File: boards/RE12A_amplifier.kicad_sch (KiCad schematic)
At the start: 14 parts, among them J14 RE12A, J15 Conn_01x03 encoder_direct, Q1 NPN, U3 MOUDLE-SEEEDUINO-XIAO-ESP32C3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, U7 LM397

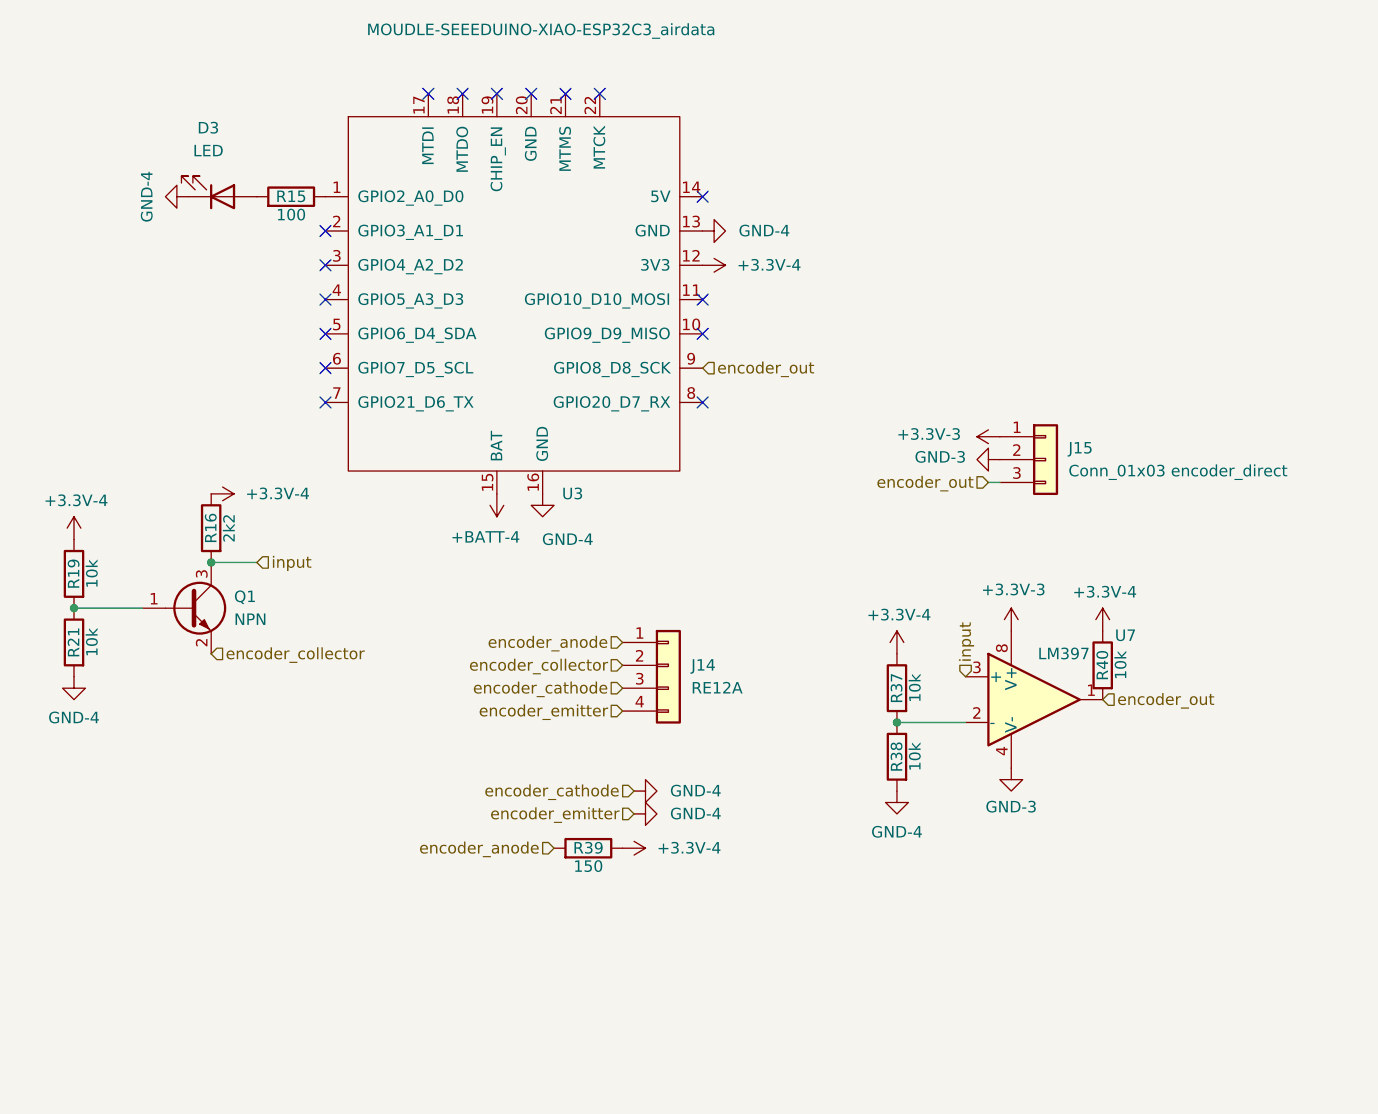
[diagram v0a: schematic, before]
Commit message: DRCエラー解消
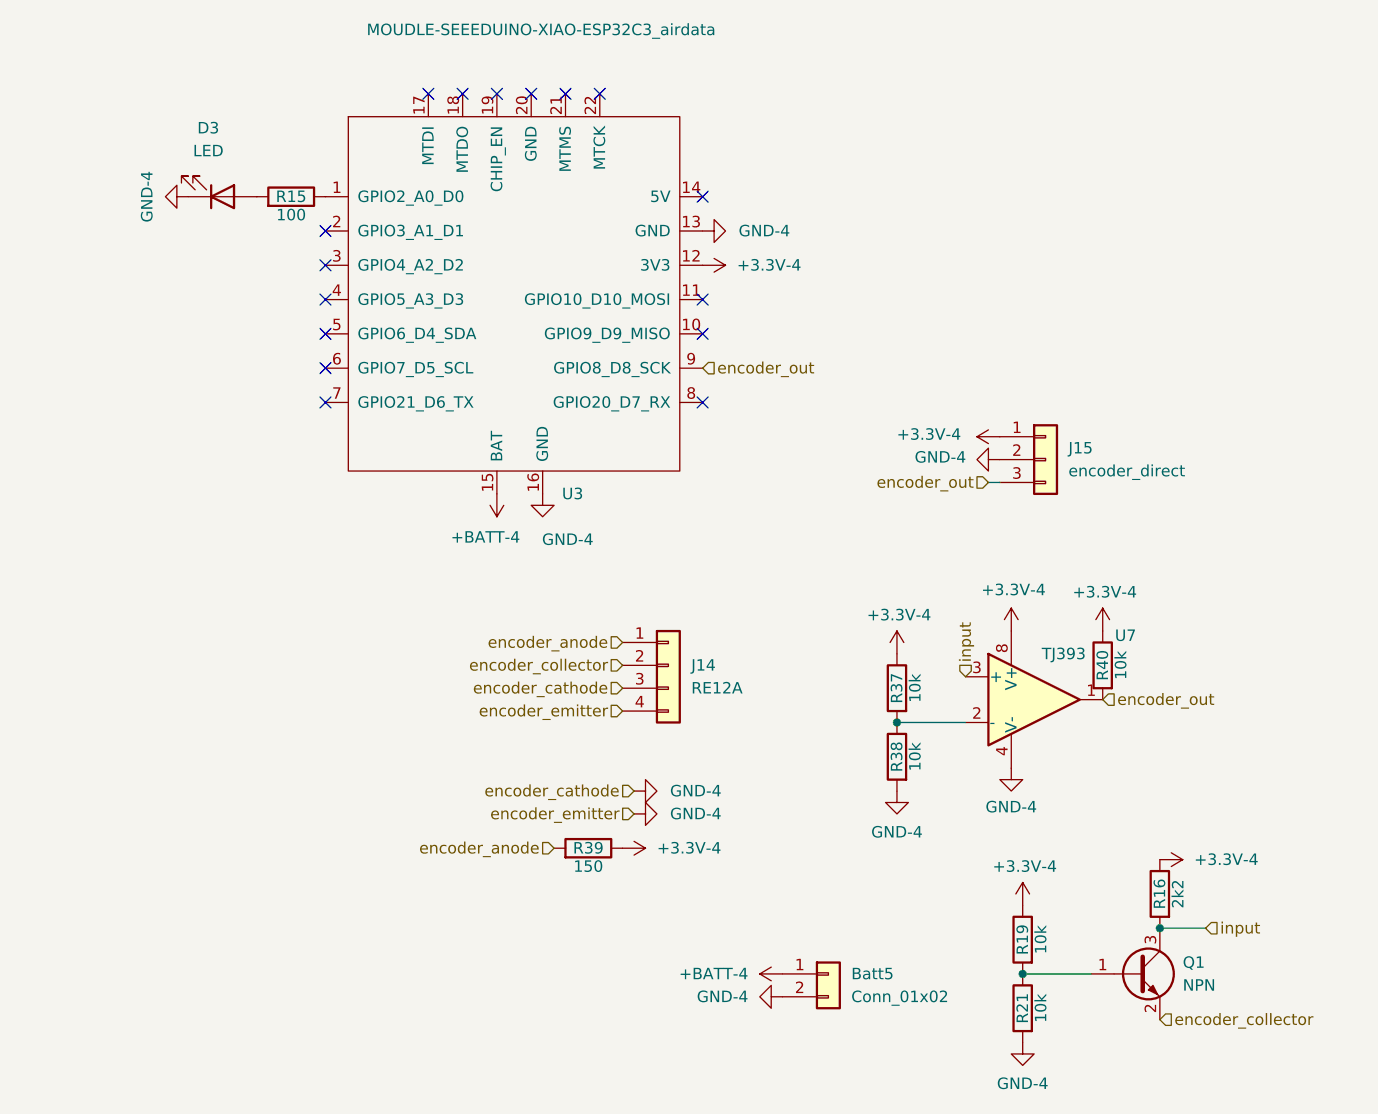
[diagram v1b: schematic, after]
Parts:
- added Batt5: Conn_01x02, Connector_JST:JST_PH_S2B-PH-SM4-TB_1x02-1MP_P2.00mm_Horizontal, symbol Connector_Generic:Conn_01x02
- J15: value Conn_01x03 encoder_direct -> encoder_direct
- U7: value LM397 -> TJ393
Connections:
- net +3.3V-3 is gone; now on net +3.3V-4: J15.1 (Pin_1), U7.8 (V+)
- net GND-3 is gone; now on net GND-4: J15.2 (Pin_2), U7.4 (V-)
- net +BATT-4: now also Batt5.1 (Pin_1)
- net GND-4: now also Batt5.2 (Pin_2)
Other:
- moved on the sheet: Q1, R16, R19, R21
